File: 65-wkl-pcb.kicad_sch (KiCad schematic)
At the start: 168 parts, among them J1 USB_C_Receptacle_USB2.0_16P, J2 Conn_01x04, J3 Conn_01x05, U1 XC6206PxxxMR, U2 SRV05-4, U3 RP2040, U4 W25Q128JVS, Y1 Crystal_GND24

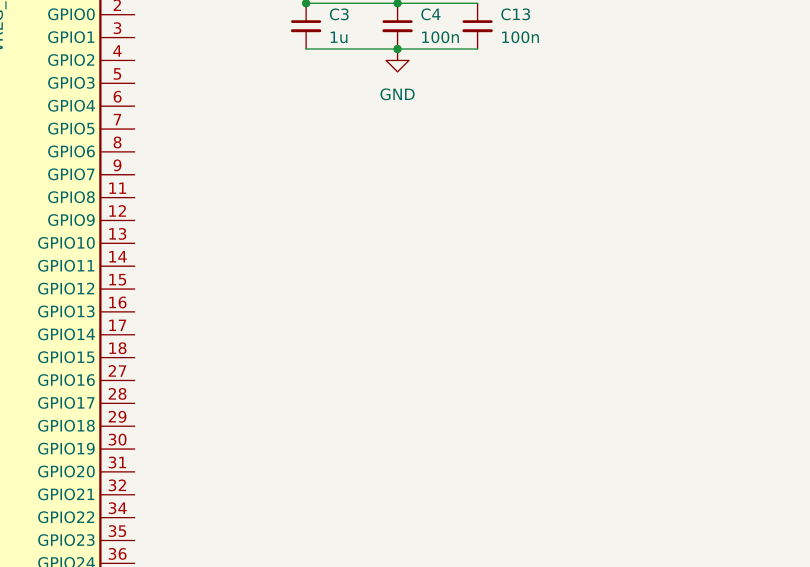
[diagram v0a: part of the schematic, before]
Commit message: updating
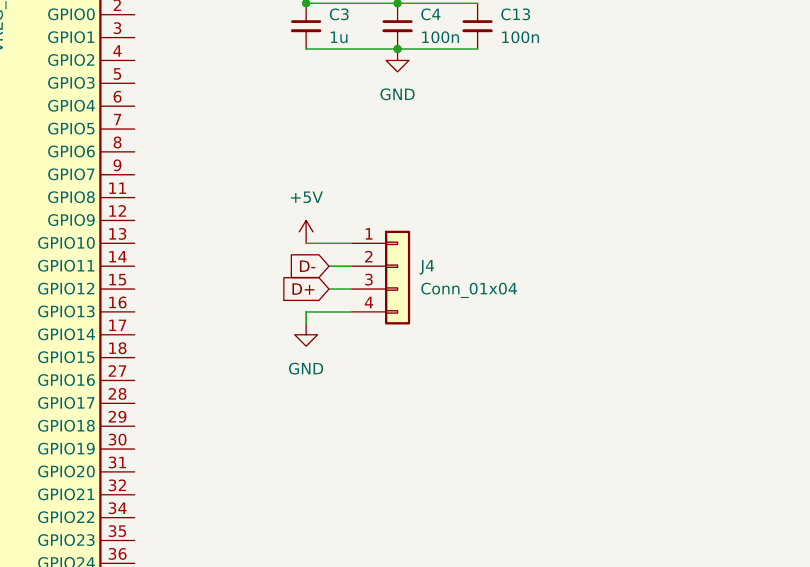
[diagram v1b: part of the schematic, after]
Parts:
- added J4: Conn_01x04, Connector_JST:JST_PH_S4B-PH-K_1x04_P2.00mm_Horizontal, symbol Connector_Generic:Conn_01x04
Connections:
- net +5V: now also J4.1 (Pin_1)
- net D+: now also J4.3 (Pin_3)
- net D-: now also J4.2 (Pin_2)
- net GND: now also J4.4 (Pin_4)

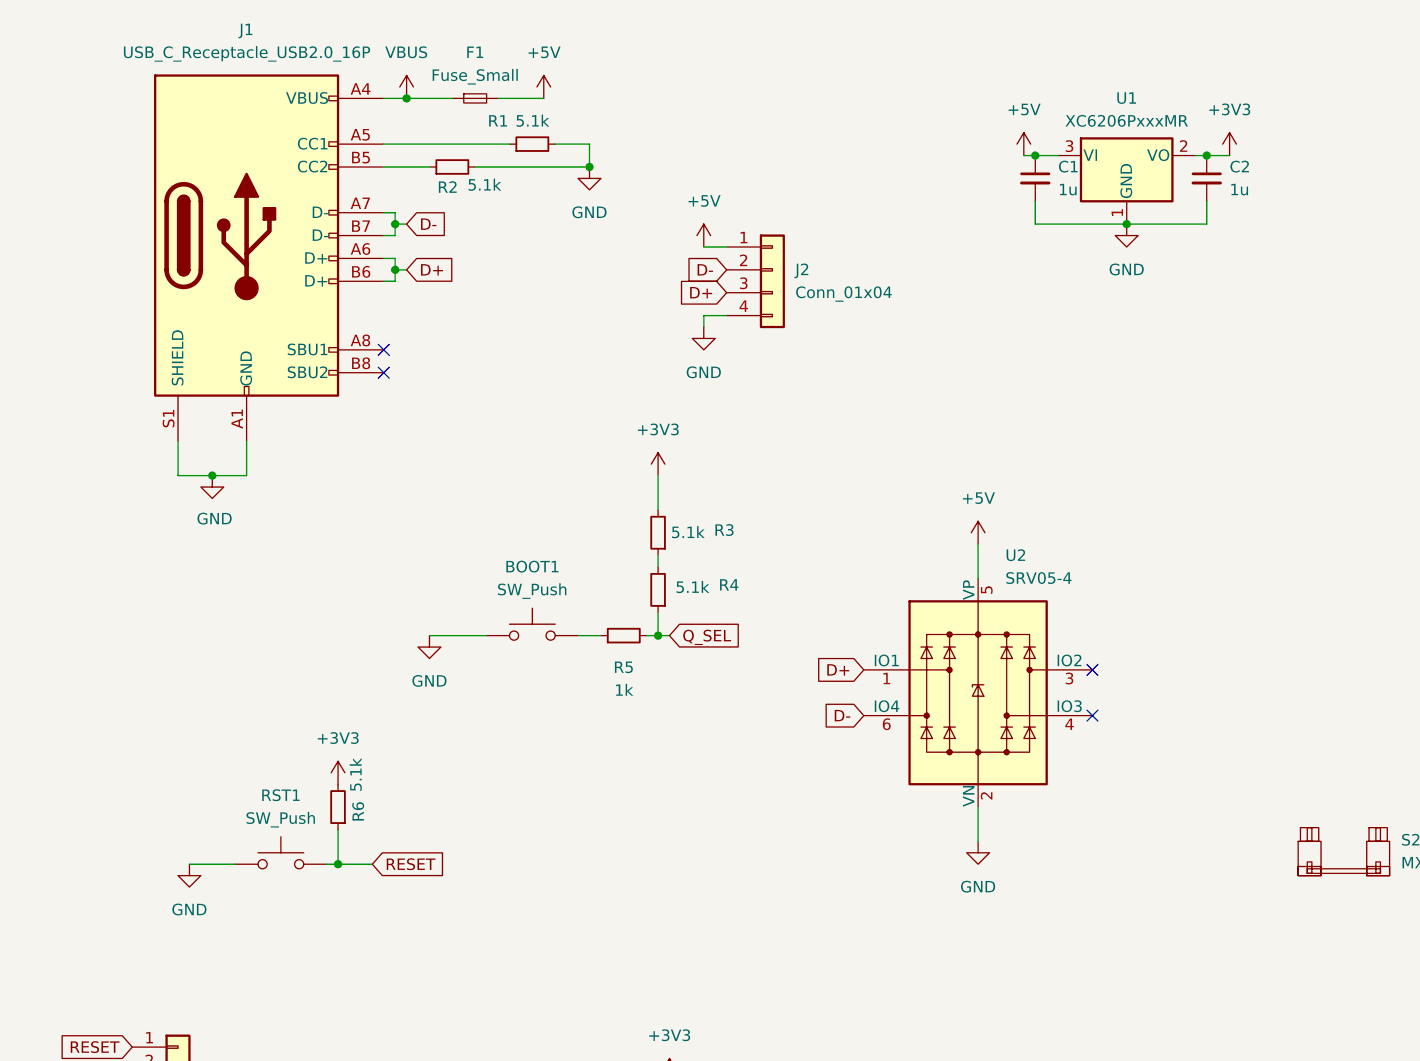
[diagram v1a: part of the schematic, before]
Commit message: daughterboard
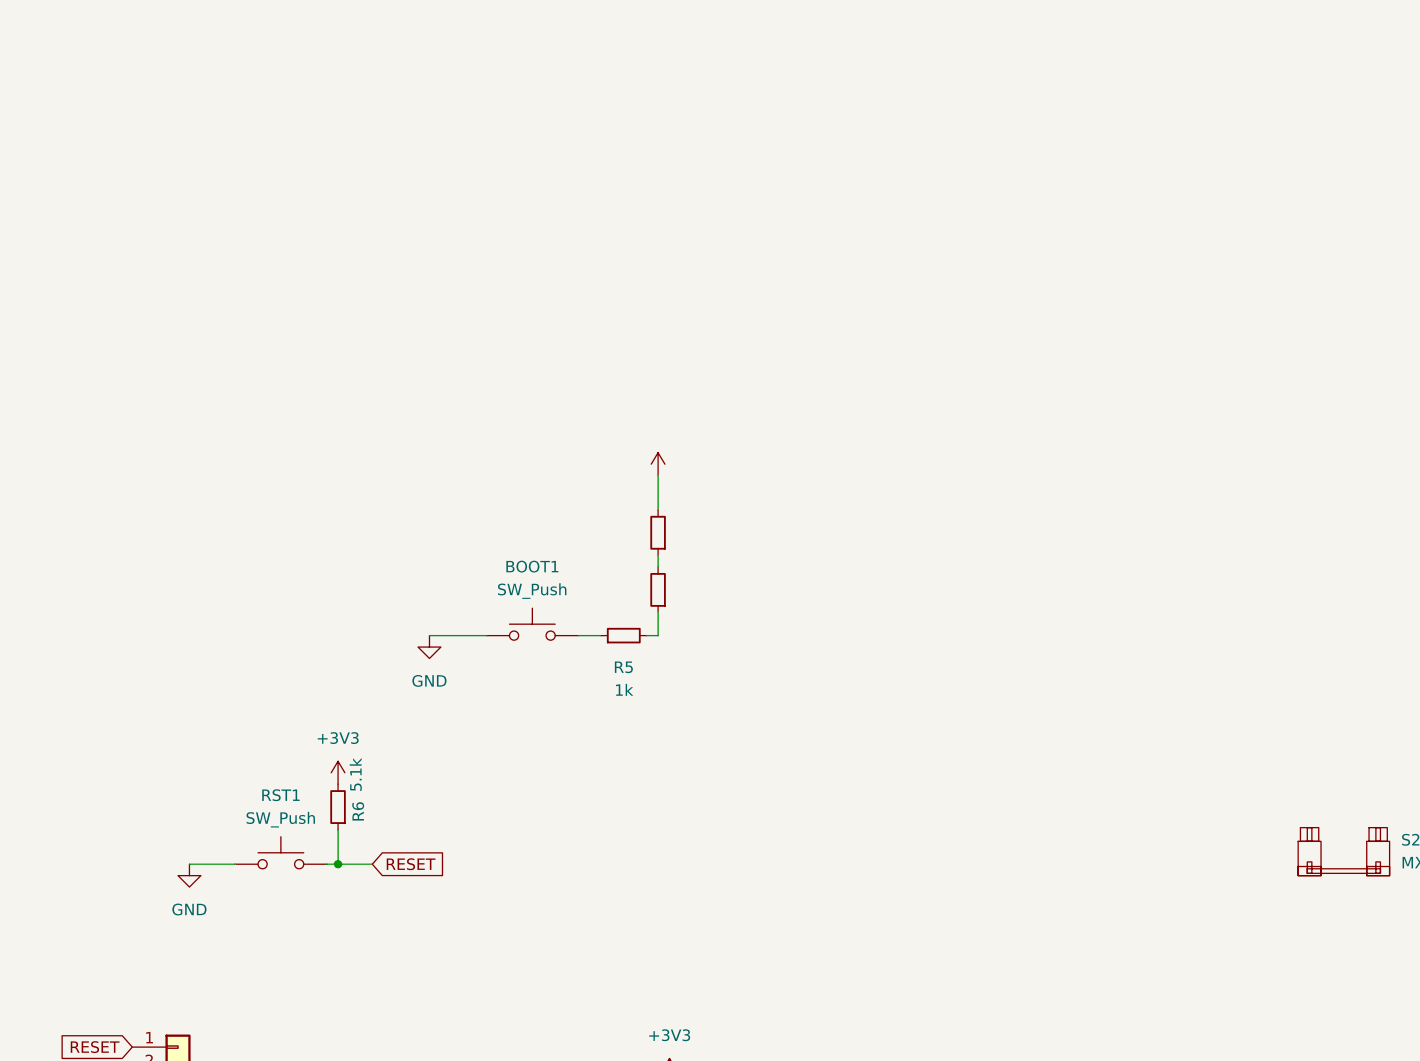
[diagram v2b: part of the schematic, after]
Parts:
- removed C1, C2: 1u, Capacitor_SMD:C_0402_1005Metric, symbol Device:C_Small
- removed F1: Fuse_Small, Fuse:Fuse_1206_3216Metric, symbol Device:Fuse_Small
- removed J1: USB_C_Receptacle_USB2.0_16P, Connector_USB:USB_C_Receptacle_HRO_TYPE-C-31-M-12, symbol Connector:USB_C_Receptacle_USB2.0_16P
- removed J2: Conn_01x04, Connector_JST:JST_PH_S4B-PH-K_1x04_P2.00mm_Horizontal, symbol Connector_Generic:Conn_01x04
- removed R1, R2: 5.1k, Resistor_SMD:R_0402_1005Metric, symbol Device:R_Small
- removed U1: XC6206PxxxMR, Package_TO_SOT_SMD:SOT-23-3, symbol Regulator_Linear:XC6206PxxxMR
- removed U2: SRV05-4, PCM_marbastlib-various:SOT-23-6-routable, symbol PCM_marbastlib-various:SRV05-4
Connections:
- net Q_SEL: no longer R4.1, R5.2
- new net: R4.1, R5.2
- no-connect marks 4 -> 0
